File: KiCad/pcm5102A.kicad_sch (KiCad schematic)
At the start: 1 part, among them U1 PCM5102A

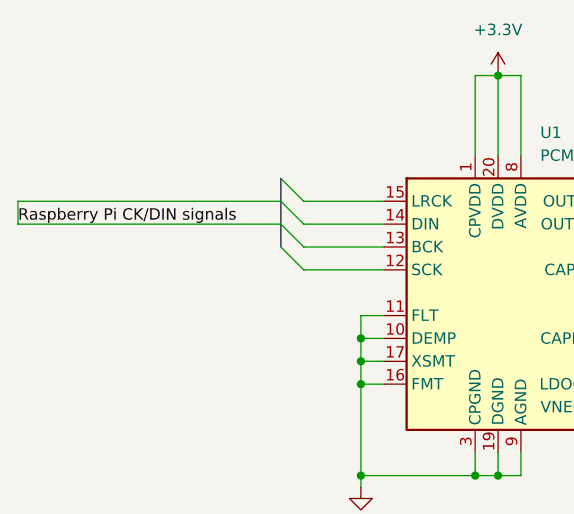
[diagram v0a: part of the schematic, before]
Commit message: First PCB layout iteration, custom footprint for Pico
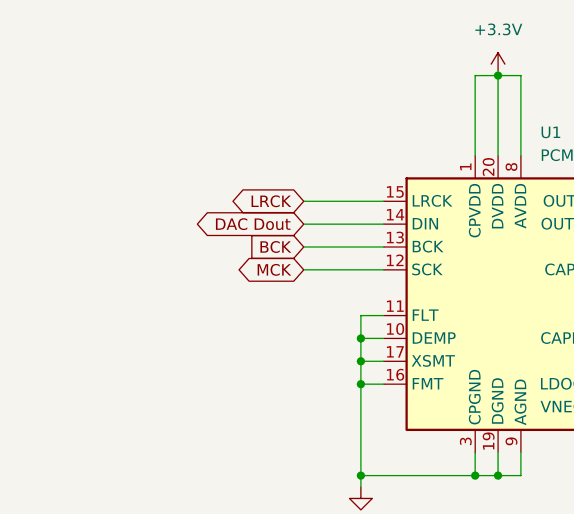
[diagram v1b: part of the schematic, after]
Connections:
- net MCK: now reaches U1.12 (SCK)
- net BCK: now reaches U1.13 (BCK)
- net DAC Dout: now reaches U1.14 (DIN)
- net LRCK: now reaches U1.15 (LRCK)
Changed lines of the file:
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@@
-		)
-	)
-	(bus_entry
-		(at 119.38 83.82)
-		(size -2.54 -2.54)
-		(stroke
-			(width 0)
-			(type default)
-		)
-	)
-	(bus_entry
-		(at 116.84 76.2)
-		(size 2.54 2.54)
-		(stroke
-			(width 0)
-			(type default)
-		)
-	)
-	(bus_entry
-		(at 119.38 81.28)
-		(size -2.54 -2.54)
-		(stroke
-			(width 0)
-			(type default)
-		)
-	)
-	(bus_entry
-		(at 119.38 86.36)
-		(size -2.54 -2.54)
-		(stroke
-			(width 0)
-			(type default)
 		)
 	)
@@
 	(wire
 		(pts
-			(xy 116.84 78.74) (xy 87.63 78.74)
-		)
-		(stroke
-			(width 0)
-			(type default)
-		)
-	)
-	(wire
-		(pts
 			(xy 125.73 99.06) (xy 125.73 109.22)
 		)
@@
 		)
 	)
+	(wire
+		(pts
+			(xy 125.73 99.06) (xy 128.27 99.06)
+		)
+		(stroke
+			(width 0)
+			(type default)
+		)
+	)
+	(wire
+		(pts
+			(xy 125.73 109.22) (xy 125.73 110.49)
+		)
+		(stroke
+			(width 0)
+			(type default)
+		)
+	)
+	(wire
+		(pts
+			(xy 153.67 81.28) (xy 163.83 81.28)
+		)
+		(stroke
+			(width 0)
+			(type default)
+		)
+	)
+	(wire
+		(pts
+			(xy 125.73 93.98) (xy 128.27 93.98)
+		)
+		(stroke
+			(width 0)
+			(type default)
+		)
+	)
+	(wire
+		(pts
+			(xy 138.43 106.68) (xy 138.43 109.22)
+		)
+		(stroke
+			(width 0)
+			(type default)
+		)
+	)
+	(wire
+		(pts
+			(xy 153.67 78.74) (xy 163.83 78.74)
+		)
+		(stroke
+			(width 0)
+			(type default)
+		)
+	)
+	(wire
+		(pts
+			(xy 187.96 78.74) (xy 187.96 76.2)
+		)
+		(stroke
+			(width 0)
+			(type default)
+		)
+	)
+	(wire
+		(pts
+			(xy 128.27 91.44) (xy 125.73 91.44)
+		)
+		(stroke
+			(width 0)
+			(type default)
+		)
+	)
+	(wire
+		(pts
+			(xy 140.97 64.77) (xy 138.43 64.77)
+		)
+		(stroke
+			(width 0)
+			(type default)
+		)
+	)
+	(wire
+		(pts
+			(xy 125.73 96.52) (xy 128.27 96.52)
+		)
+		(stroke
+			(width 0)
+			(type default)
+		)
+	)
+	(wire
+		(pts
+			(xy 125.73 91.44) (xy 125.73 93.98)
+		)
+		(stroke
+			(width 0)
+			(type default)
+		)
+	)
+	(wire
+		(pts
+			(xy 140.97 64.77) (xy 143.51 64.77)
+		)
+		(stroke
+			(width 0)
+			(type default)
+		)
+	)
+	(wire
+		(pts
+			(xy 119.38 81.28) (xy 128.27 81.28)
+		)
+		(stroke
+			(width 0)
+			(type default)
+		)
+	)
+	(wire
+		(pts
+			(xy 138.43 64.77) (xy 138.43 73.66)
+		)
+		(stroke
+			(width 0)
+			(type default)
+		)
+	)
 	(bus
 		(pts
-			(xy 116.84 76.2) (xy 116.84 83.82)
-		)
-		(stroke
-			(width 0)
-			(type default)
-		)
-	)
-	(wire
-		(pts
-			(xy 125.73 99.06) (xy 128.27 99.06)
-		)
-		(stroke
-			(width 0)
-			(type default)
-		)
-	)
-	(wire
-		(pts
-			(xy 125.73 109.22) (xy 125.73 110.49)
-		)
-		(stroke
-			(width 0)
-			(type default)
-		)
-	)
-	(wire
-		(pts
-			(xy 153.67 81.28) (xy 163.83 81.28)
-		)
-		(stroke
-			(width 0)
-			(type default)
-		)
-	)
-	(wire
-		(pts
-			(xy 125.73 93.98) (xy 128.27 93.98)
-		)
-		(stroke
-			(width 0)
-			(type default)
-		)
-	)
-	(wire
-		(pts
-			(xy 138.43 106.68) (xy 138.43 109.22)
-		)
-		(stroke
-			(width 0)
-			(type default)
-		)
-	)
-	(wire
-		(pts
-			(xy 153.67 78.74) (xy 163.83 78.74)
-		)
-		(stroke
-			(width 0)
-			(type default)
-		)
-	)
-	(wire
-		(pts
-			(xy 187.96 78.74) (xy 187.96 76.2)
-		)
-		(stroke
-			(width 0)
-			(type default)
-		)
-	)
-	(wire
-		(pts
-			(xy 128.27 91.44) (xy 125.73 91.44)
-		)
-		(stroke
-			(width 0)
-			(type default)
-		)
-	)
-	(wire
-		(pts
-			(xy 87.63 81.28) (xy 116.84 81.28)
-		)
-		(stroke
-			(width 0)
-			(type default)
-		)
-	)
-	(wire
-		(pts
-			(xy 140.97 64.77) (xy 138.43 64.77)
-		)
-		(stroke
-			(width 0)
-			(type default)
-		)
-	)
-	(wire
-		(pts
-			(xy 125.73 96.52) (xy 128.27 96.52)
-		)
-		(stroke
-			(width 0)
-			(type default)
-		)
-	)
-	(wire
-		(pts
-			(xy 125.73 91.44) (xy 125.73 93.98)
-		)
-		(stroke
-			(width 0)
-			(type default)
-		)
-	)
-	(wire
-		(pts
-			(xy 140.97 64.77) (xy 143.51 64.77)
-		)
-		(stroke
-			(width 0)
-			(type default)
-		)
-	)
-	(wire
-		(pts
-			(xy 119.38 81.28) (xy 128.27 81.28)
-		)
-		(stroke
-			(width 0)
-			(type default)
-		)
-	)
-	(wire
-		(pts
-			(xy 138.43 64.77) (xy 138.43 73.66)
-		)
-		(stroke
-			(width 0)
-			(type default)
-		)
-	)
-	(wire
-		(pts
-			(xy 87.63 78.74) (xy 87.63 81.28)
-		)
-		(stroke
-			(width 0)
-			(type default)
-		)
-	)
-	(bus
-		(pts
 			(xy 166.37 76.2) (xy 166.37 78.74)
 		)
@@
 			(width 0)
 			(type default)
-		)
-	)
-	(label "Raspberry Pi CK{slash}DIN signals"
-		(at 87.63 81.28 0)
-		(effects
-			(font
-				(size 1.27 1.27)
-			)
-			(justify left bottom)
 		)
 	)
@@
 		)
 	)
+	(global_label "DAC Dout"
+		(shape bidirectional)
+		(at 119.38 81.28 180)
+		(effects
+			(font
+				(size 1.27 1.27)
+			)
+			(justify right)
+		)
+		(property "Intersheetrefs" "${INTERSHEET_REFS}"
+			(at 119.38 81.28 0)
+			(hide yes)
+			(show_name no)
+			(do_not_autoplace no)
+			(effects
+				(font
+					(size 1.27 1.27)
+				)
+			)
+		)
+	)
+	(global_label "MCK"
+		(shape bidirectional)
+		(at 119.38 86.36 180)
+		(effects
+			(font
+				(size 1.27 1.27)
+			)
+			(justify right)
+		)
+		(property "Intersheetrefs" "${INTERSHEET_REFS}"
+			(at 119.38 86.36 0)
+			(hide yes)
+			(show_name no)
+			(do_not_autoplace no)
+			(effects
+				(font
+					(size 1.27 1.27)
+				)
+			)
+		)
+	)
+	(global_label "LRCK"
+		(shape bidirectional)
+		(at 119.38 78.74 180)
+		(effects
+			(font
+				(size 1.27 1.27)
+			)
+			(justify right)
+		)
+		(property "Intersheetrefs" "${INTERSHEET_REFS}"
+			(at 119.38 78.74 0)
+			(hide yes)
+			(show_name no)
+			(do_not_autoplace no)
+			(effects
+				(font
+					(size 1.27 1.27)
+				)
+			)
+		)
+	)
+	(global_label "BCK"
+		(shape input)
+		(at 119.38 83.82 180)
+		(fields_autoplaced yes)
+		(effects
+			(font
+				(size 1.27 1.27)
+			)
+			(justify right)
+		)
+		(property "Intersheetrefs" "${INTERSHEET_REFS}"
+			(at 112.5848 83.82 0)
+			(hide yes)
+			(show_name no)
+			(do_not_autoplace no)
+			(effects
+				(font
+					(size 1.27 1.27)
+				)
+				(justify right)
+			)
+		)
+	)

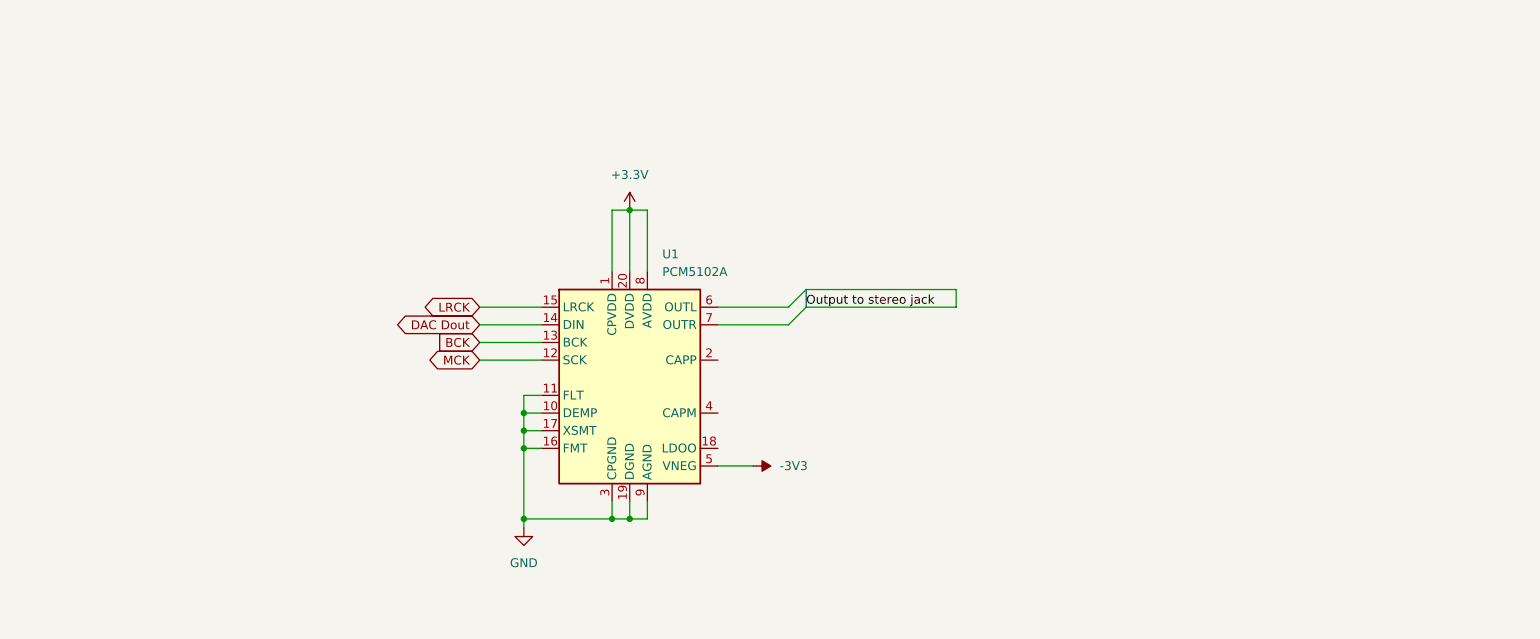
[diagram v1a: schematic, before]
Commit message: Changed footprints, added powersystem
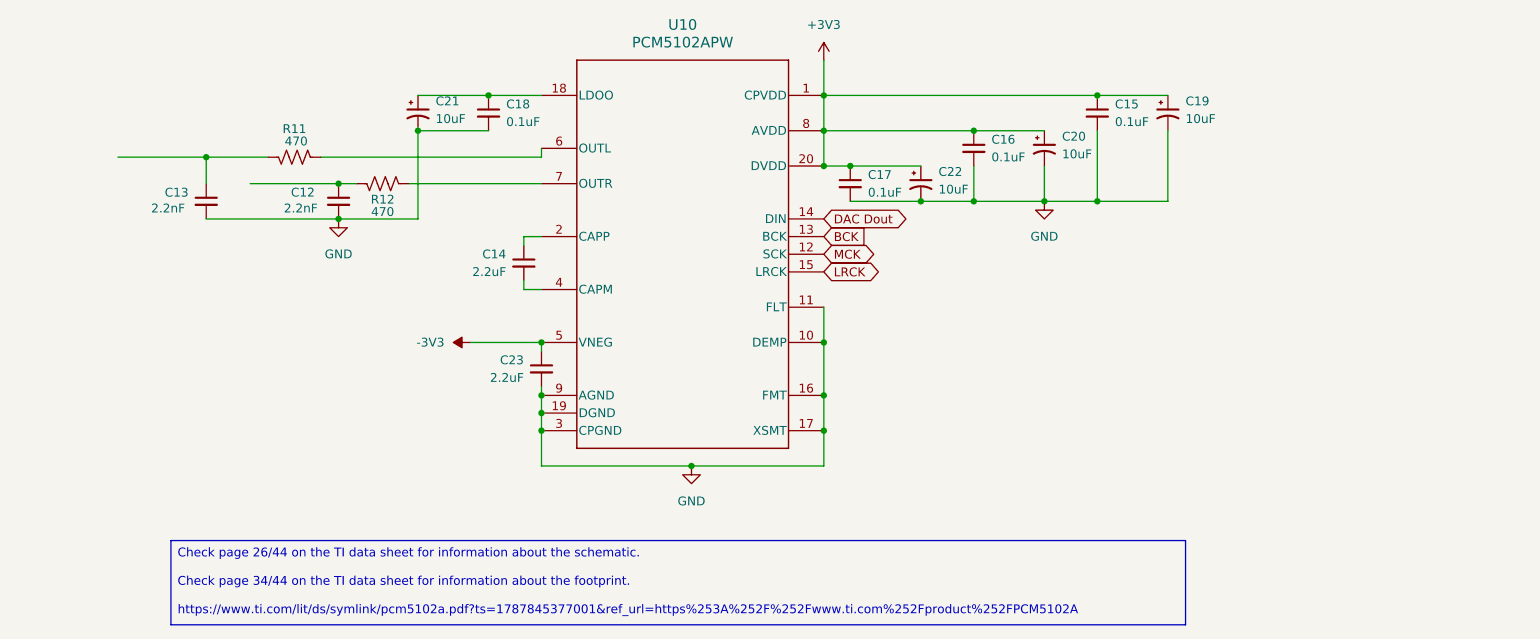
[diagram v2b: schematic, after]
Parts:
- removed U1: PCM5102A, Package_SO:TSSOP-20_4.4x6.5mm_P0.65mm, symbol Audio:PCM5102A
- added C12, C13: 2.2nF, Capacitor_SMD:C_0402_1005Metric, symbol Device:C_Small
- added C14, C23: 2.2uF, Capacitor_SMD:C_0603_1608Metric, symbol Device:C_Small
- added C15, C16, C17, C18: 0.1uF, Capacitor_SMD:C_0603_1608Metric, symbol Device:C_Small
- added C19, C20, C21, C22: 10uF, Capacitor_SMD:CP_Elec_6.3x5.4, symbol Device:C_Polarized_Small_US
- added R11, R12: 470, Resistor_SMD:R_1206_3216Metric, symbol Device:R_US
- added U10: PCM5102APW, PW0020A_N, symbol DAC:PCM5102APW
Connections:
- net -3V3: now also C23.1, U10.5 (VNEG)
- net BCK: now also U10.13 (BCK)
- net DAC Dout: now also U10.14 (DIN)
- net GND: now also C12.2, C13.2, C15.2, C16.2, C17.2, C18.2, C19.2, C20.2, C21.2, C22.2, C23.2, U10.10 (DEMP), U10.11 (FLT), U10.16 (FMT), U10.17 (XSMT), U10.19 (DGND), U10.3 (CPGND), U10.9 (AGND)
- net LRCK: now also U10.15 (LRCK)
- net MCK: now also U10.12 (SCK)
- new net: R11.1, U10.6 (OUTL)
- new net: C13.1, R11.2
- new net: C12.1, R12.2
- new net: C18.1, C21.1, U10.18 (LDOO)
- new net: C14.1, U10.2 (CAPP)
- new net: C14.2, U10.4 (CAPM)
- new net: R12.1, U10.7 (OUTR)
- new net +3V3: C15.1, C16.1, C17.1, C19.1, C20.1, C22.1, U10.1 (CPVDD), U10.20 (DVDD), U10.8 (AVDD)

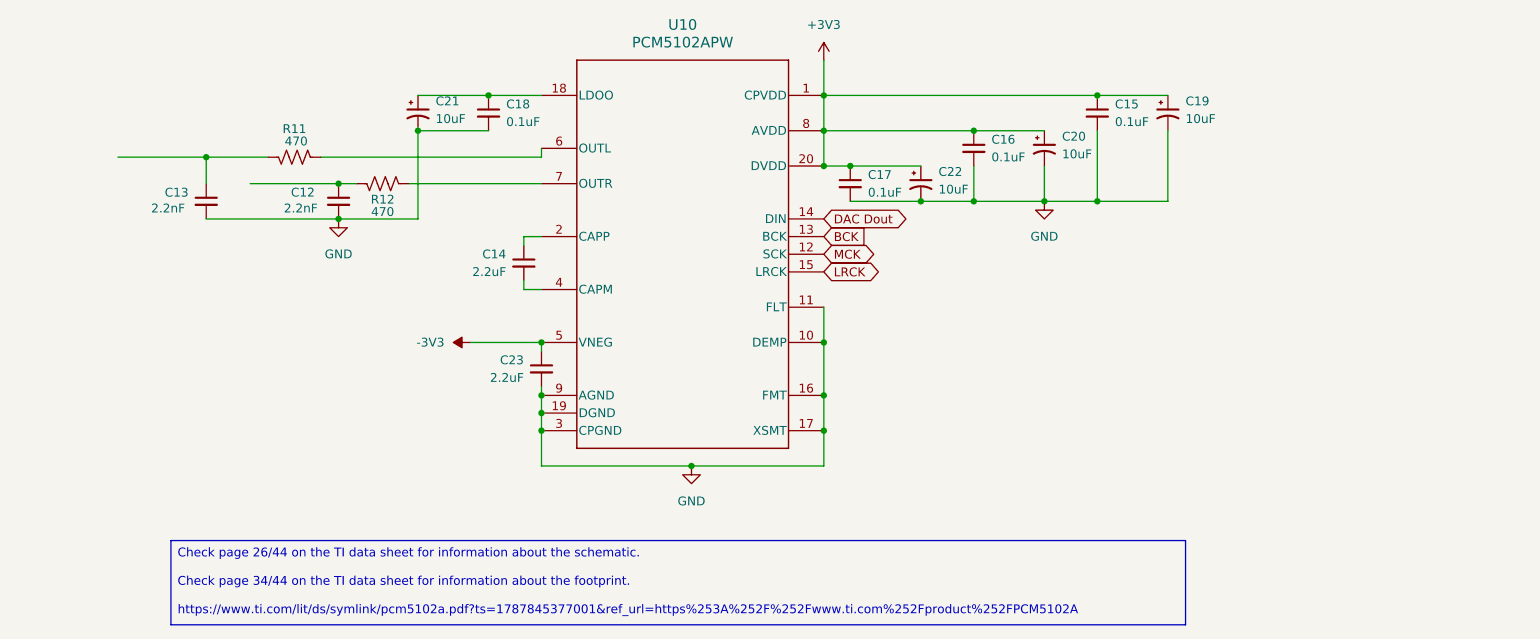
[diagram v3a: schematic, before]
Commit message: Pushing PCB, and controls schem
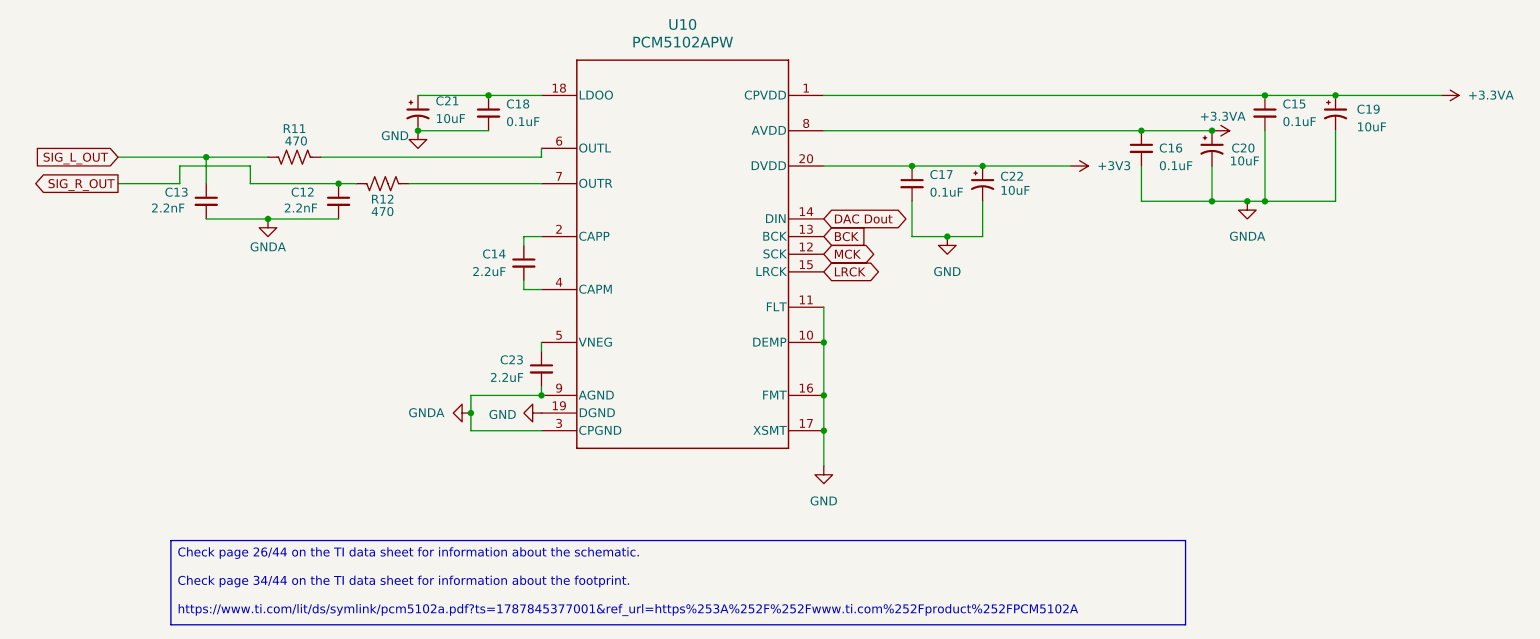
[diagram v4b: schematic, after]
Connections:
- net +3V3: no longer C15.1, C16.1, C19.1, C20.1, U10.1 (CPVDD), U10.8 (AVDD)
- net GND: no longer C12.2, C13.2, C15.2, C16.2, C19.2, C20.2, C23.2, U10.3 (CPGND), U10.9 (AGND)
- net SIG_L_OUT: now reaches C13.1, R11.2
- net SIG_R_OUT: now reaches C12.1, R12.2
- net -3V3: no longer names the net of C23.1, U10.5 (VNEG)
- new net +3.3VA: C15.1, C16.1, C19.1, C20.1, U10.1 (CPVDD), U10.8 (AVDD)
- new net GNDA: C12.2, C13.2, C15.2, C16.2, C19.2, C20.2, C23.2, U10.3 (CPGND), U10.9 (AGND)
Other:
- moved on the sheet: C15, C16, C17, C19, C20, C22

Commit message: PCB ex
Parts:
- U10: footprint PW0020A_N -> Package_SO:Texas_PW0020A_TSSOP-20_4.4x6.5mm_P0.65mm
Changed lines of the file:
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@@
 			)
 		)
-		(property "Footprint" "PW0020A_N"
+		(property "Footprint" "Package_SO:Texas_PW0020A_TSSOP-20_4.4x6.5mm_P0.65mm"
 			(at 148.336 45.212 0)
 			(hide yes)
